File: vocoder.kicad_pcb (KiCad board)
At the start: 4 copper layers, 65.4 x 35.6 mm, 66 parts, among them J1 AudioJack4, J2 Conn_01x02_Socket, J3 Conn_01x02_Pin, J4 USB_C_Receptacle_USB2.0_16P, Q1 Q_NPN_BCE, Q2 Q_NPN_BCE, Q3 AO3401A, Q4 Q_NPN_BCE, SW1 SW_SPDT, SW2 SW_Push, SW3 SW_Push, U2 MAX98357A, U3 BQ24074RGT, U4 TPS63031DSK, U5 ADAU1761, U7 ESP32-S3-WROOM-1

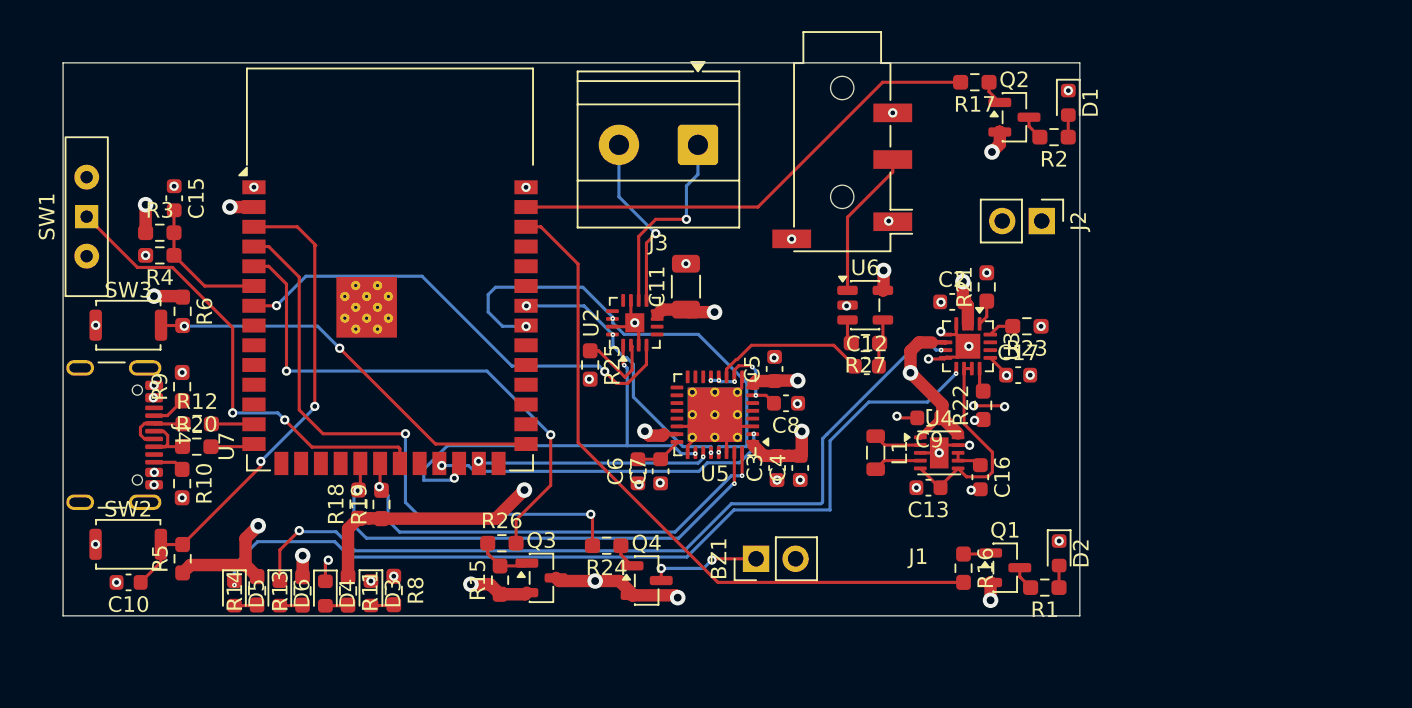
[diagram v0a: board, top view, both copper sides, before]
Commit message: semi working before removing battery and adding necessary changes
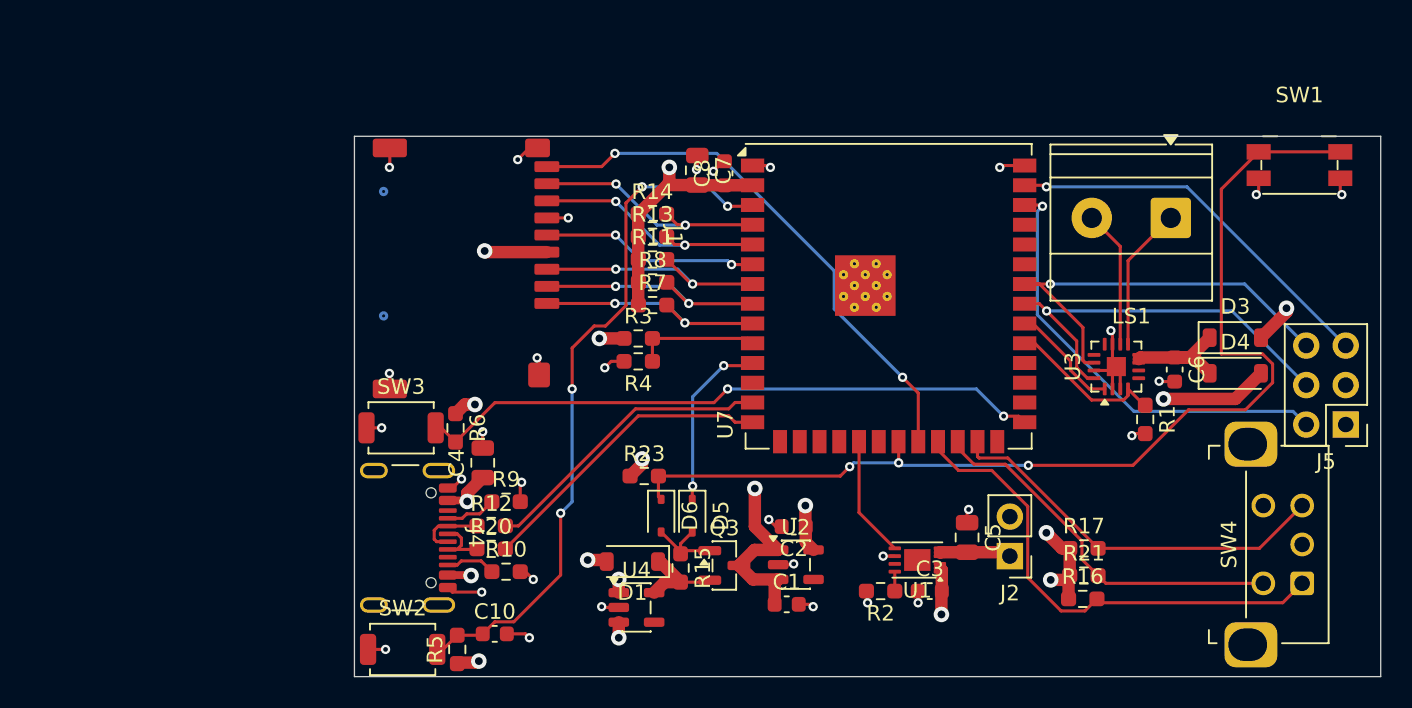
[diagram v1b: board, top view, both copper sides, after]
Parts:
- removed BZ1: Buzzer, Connector_PinHeader_2.54mm:PinHeader_1x02_P2.54mm_Vertical
- removed C11: 220u, Capacitor_SMD:C_1206_3216Metric
- removed C12: 2.2u, Capacitor_SMD:C_0603_1608Metric
- removed C13, C17, C9: 10u, Capacitor_SMD:C_0603_1608Metric
- removed C15: 100n, Capacitor_SMD:C_0603_1608Metric
- removed C16: 0.1u, Capacitor_SMD:C_0603_1608Metric
- removed D2: LED RED, LED_SMD:LED_0603_1608Metric
- removed J3: Conn_01x02_Pin, TerminalBlock_Phoenix:TerminalBlock_Phoenix_MKDS-1,5-2-5.08_1x02_P5.08mm_Horizontal
- removed L1: 1.5uH, Inductor_SMD:L_0805_2012Metric
- removed Q1, Q2, Q4: Q_NPN_BCE, Package_TO_SOT_SMD:SOT-23
- removed R18, R19: 10k, Resistor_SMD:R_0603_1608Metric_Pad0.98x0.95mm_HandSolder
- removed R22, R24: 1k, Resistor_SMD:R_0603_1608Metric_Pad0.98x0.95mm_HandSolder
- removed R25: 100k, Resistor_SMD:R_0603_1608Metric_Pad0.98x0.95mm_HandSolder
- removed R26: 100, Resistor_SMD:R_0603_1608Metric_Pad0.98x0.95mm_HandSolder
- removed R27: 51, Resistor_SMD:R_0603_1608Metric_Pad0.98x0.95mm_HandSolder
- removed U5: ADAU1761, Package_CSP:LFCSP-32-1EP_5x5mm_P0.5mm_EP3.5x3.5mm_ThermalVias
- removed U6: ~, custom_footprints:TLV9041
- added C1: 1u, Capacitor_SMD:C_0603_1608Metric, F.Cu at (169.6, 101.6)
- added J5: Conn_02x03_Top_Bottom, Connector_PinHeader_2.54mm:PinHeader_2x03_P2.54mm_Vertical, F.Cu at (205.5, 90.0)
- added LS1: Speaker, TerminalBlock_Phoenix:TerminalBlock_Phoenix_MKDS-1,5-2-5.08_1x02_P5.08mm_Horizontal, F.Cu at (194.2, 76.8)
- added R7: 10k, Resistor_SMD:R_0603_1608Metric_Pad0.98x0.95mm_HandSolder, F.Cu at (160.9, 82.4)
- added SW4: RotaryEncoder_Switch, Rotary_Encoder:RotaryEncoder_Bourns_Horizontal_PEC12R-2x17F-Sxxxx, F.Cu at (202.7, 100.2)
- added U1: MCP73831-2-MC, Package_DFN_QFN:DFN-8-1EP_3x2mm_P0.5mm_EP1.7x1.4mm, F.Cu at (177.9, 98.8)
- C2, C8: value 10u -> 1u
- C3, C6: value 100n -> 1u
- C4, C7: footprint Capacitor_SMD:C_0603_1608Metric -> Capacitor_SMD:C_0805_2012Metric
- C5: value 100n -> 10u; footprint Capacitor_SMD:C_0603_1608Metric -> Capacitor_SMD:C_0805_2012Metric
- D1: value LED RED -> SS34; footprint LED_SMD:LED_0603_1608Metric -> Diode_SMD:D_SOD-123
- D3: value LED BLUE -> SS34; footprint LED_SMD:LED_0603_1608Metric -> Diode_SMD:D_SOD-123
- D4: value LED GREEN -> SS34; footprint LED_SMD:LED_0603_1608Metric -> Diode_SMD:D_SOD-123
- D5: value LED RED -> 1N4148; footprint LED_SMD:LED_0603_1608Metric -> Diode_SMD:D_SOD-323
- D6: value LED GREEN -> 1N4148; footprint LED_SMD:LED_0603_1608Metric -> Diode_SMD:D_SOD-323
- J1: value AudioJack4 -> Micro_SD_Card_Det1; footprint Connector_Audio:Jack_3.5mm_PJ320D_Horizontal -> MyAntenna_manufacturer:Untitled
- R1, R11, R13, R14, R16, R17, R23, R8: value 1k -> 10k
- R2: value 1k -> 2.2k
- R3, R4: value 100k -> 470k
- SW1: value SW_SPDT -> SW_Push; footprint Button_Switch_THT:SW_Slide-03_Wuerth-WS-SLTV_10x2.5x6.4_P2.54mm -> Button_Switch_SMD:Panasonic_EVQPUJ_EVQPUA
- SW2, SW3: footprint Button_Switch_SMD:SW_Push_SPST_NO_Alps_SKRK -> Button_Switch_SMD:SW_SPST_TS-1088-xR020
- U2: value MAX98357A -> AP2112K-3.3; footprint Package_DFN_QFN:TQFN-16-1EP_3x3mm_P0.5mm_EP1.23x1.23mm -> Package_TO_SOT_SMD:SOT-23-5
- U3: value BQ24074RGT -> MAX98357A; footprint Package_DFN_QFN:VQFN-16-1EP_3x3mm_P0.5mm_EP1.6x1.6mm -> Package_DFN_QFN:TQFN-16-1EP_3x3mm_P0.5mm_EP1.23x1.23mm
- U4: value TPS63031DSK -> MAX40200AUK; footprint Package_SON:WSON-10-1EP_2.5x2.5mm_P0.5mm_EP1.2x2mm -> Package_TO_SOT_SMD:SOT-23-5
- U7: footprint RF_Module:ESP32-S3-WROOM-1 -> RF_Module:ESP32-S3-WROOM-1U
- moved SW1 78.1 mm to (202.5, 73.3), turned to 0 degrees
- moved D4 60.2 mm to (198.4, 86.7), turned to 0 degrees
- moved D3 58.0 mm to (198.4, 84.5), turned to 0 degrees
- moved D1 40.7 mm to (159.6, 98.8), turned to 180 degrees
- moved C6 35.1 mm to (194.5, 86.5), turned to -90 degrees
- moved R14 35.1 mm to (160.9, 76.5), turned to 0 degrees
- moved U7 32.1 mm to (176.1, 81.8)
- moved R13 32.0 mm to (160.9, 78.0), turned to 0 degrees
- moved R4 31.5 mm to (160.0, 86.0)
- moved R3 31.5 mm to (160.0, 84.5)
- moved R2 31.3 mm to (175.6, 100.8)
- moved R17 30.8 mm to (188.7, 98.0), turned to 0 degrees
- moved D5 29.9 mm to (163.5, 95.9)
- moved R11 28.9 mm to (160.9, 79.4), turned to 0 degrees
- moved R23 26.4 mm to (160.4, 93.3), turned to 0 degrees
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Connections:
- C2 pad 1: GND -> 3V3
- C2 pad 2: BATT+ -> GND
- C3 pad 2: 3V3 -> USB_5V
- C4 pad 1: GND -> USB_5V
- C4 pad 2: 3V3 -> GND
- C5 pad 1: 3V3 -> GND
- C5 pad 2: GND -> BATT+
- C6 pad 1: GND -> Net-(D3-K)
- C6 pad 2: Net-(U5-DVDDOUT) -> GND
- C7 pad 2: Net-(U5-DVDDOUT) -> 3V3
- C8 pad 1: GND -> 3V3
- C8 pad 2: CM -> GND
- D1 pad 1: GND -> Net-(D1-K)
- D1 pad 2: Net-(D1-A) -> USB_5V
- D3 pad 1: GND -> Net-(D3-K)
- D3 pad 2: Net-(D3-A) -> USB_5V
- D4 pad 1: GND -> Net-(D3-K)
- D4 pad 2: Net-(D4-A) -> AMP_POWER
- D5 pad 1: Net-(D5-K) -> POWER_SWITCH
- D6 pad 1: Net-(D6-K) -> BUTTON_READ
- D6 pad 2: Net-(D6-A) -> Net-(D5-A)
- Q3 pad 1: Net-(Q3-G) -> Net-(D5-A)
- Q3 pad 2: 3V3 -> Net-(D1-K)
- Q3 pad 3: 3V3_PRE -> AMP_POWER
- R1 pad 1: Net-(D2-A) -> AMP_SWITCH
- R1 pad 2: Net-(Q1-E) -> GND
- R11 pad 2: Net-(D4-A) -> CMD
- R13 pad 1: Net-(D6-A) -> 3V3
- R13 pad 2: 3V3_PRE -> D0
- R14 pad 1: Net-(D5-A) -> 3V3
- R14 pad 2: 3V3_PRE -> D1
- R15 pad 1: 3V3_PRE -> Net-(D5-A)
- R15 pad 2: Net-(Q3-G) -> Net-(D1-K)
- R16 pad 1: Net-(Q1-B) -> 3V3
- R16 pad 2: LED_RIGHT -> ENC_LEFT
- R17 pad 1: Net-(Q2-B) -> 3V3
- R17 pad 2: LED_LEFT -> ENC_RIGHT
- R2 pad 1: Net-(D1-A) -> Net-(U1-PROG)
- R2 pad 2: Net-(Q2-E) -> GND
- R21 pad 1: Net-(U3-TS) -> 3V3
- R21 pad 2: GND -> ENC_PUSH
- R23 pad 1: GND -> 3V3
- R23 pad 2: Net-(U3-ISET) -> BUTTON_READ
- R5 pad 1: 3V3_PRE -> 3V3
- R6 pad 1: 3V3_PRE -> 3V3
- R8 pad 1: USB_5V -> 3V3
- R8 pad 2: Net-(D3-A) -> D3
- SW1 pad 1: SWITCH_INPUT -> BUTTON_READ
- SW1 pad 2: 3V3_PRE -> GND
- U2 pad 1: I2S_DATA_OUT -> AMP_POWER
- U2 pad 2: Net-(U2-GAIN_SLOT) -> GND
- U2 pad 3: GND -> AMP_POWER
- U2 pad 4: AMP_SWITCH -> unconnected-(U2-NC-Pad4)
- U2 pad 5: unconnected-(U2-NC-Pad5) -> 3V3
- U3 pad 1: Net-(U3-TS) -> I2S_DATA_OUT
- U3 pad 10: Net-(U4-EN) -> Net-(U3-OUTN)
- U3 pad 11: Net-(U4-EN) -> GND
- U3 pad 12: Net-(U3-ILIM) -> unconnected-(U3-NC-Pad12)
- U3 pad 13: USB_5V -> unconnected-(U3-NC-Pad13)
- U3 pad 14: unconnected-(U3-TMR-Pad14) -> I2S_LRCLK
- U3 pad 15: unconnected-(U3-ITERM-Pad15) -> GND
- U3 pad 16: Net-(U3-ISET) -> I2S_BCLK
- U3 pad 2: BATT+ -> GND
- U3 pad 3: BATT+ -> GND
- U3 pad 4: GND -> AMP_SWITCH
- U3 pad 5: GND -> unconnected-(U3-NC-Pad5)
- U3 pad 6: 3V3_PRE -> unconnected-(U3-NC-Pad6)
- U3 pad 7: Net-(D6-K) -> Net-(D3-K)
- U3 pad 8: GND -> Net-(D3-K)
- U3 pad 9: Net-(D5-K) -> Net-(U3-OUTP)
- U4 pad 1: 3V3_PRE -> BATT+
- U4 pad 2: Net-(U4-L2) -> GND
- U4 pad 3: GND -> BATT+
- U4 pad 4: Net-(U4-L1) -> unconnected-(U4-NC-Pad4)
- U4 pad 5: Net-(U4-EN) -> Net-(D1-K)
- U7 pad 10: unconnected-(U7-IO17-Pad10) -> BATT_READ
- U7 pad 11: unconnected-(U7-IO18-Pad11) -> POWER_SWITCH
- U7 pad 19: SDA -> CHARGE_STATUS
- U7 pad 2: 3V3_PRE -> 3V3
- U7 pad 20: SCL -> unconnected-(U7-IO12-Pad20)
- U7 pad 21: SWITCH_INPUT -> BUTTON_READ
- U7 pad 22: unconnected-(U7-IO14-Pad22) -> DET
- U7 pad 23: I2S_MCLK -> ENC_LEFT
- U7 pad 24: I2S_DATA_OUT -> ENC_PUSH
- U7 pad 25: I2S_DATA_IN -> ENC_RIGHT
- U7 pad 31: unconnected-(U7-IO38-Pad31) -> AMP_SWITCH
- U7 pad 32: unconnected-(U7-IO39-Pad32) -> I2S_DATA_OUT
- U7 pad 33: I2S_LRCLK -> I2S_BCLK
- U7 pad 34: I2S_BCLK -> I2S_LRCLK
- U7 pad 38: LED_RIGHT -> I2S_MCLK
- U7 pad 39: LED_LEFT -> I2S_DATA_IN
- U7 pad 4: BUZZER -> D1
- U7 pad 5: 3V3_SWITCH -> D0
- U7 pad 6: BATT_READ -> CLK
- U7 pad 7: AMP_SWITCH -> CMD
- U7 pad 8: unconnected-(U7-IO15-Pad8) -> D3
- U7 pad 9: unconnected-(U7-IO16-Pad9) -> D2
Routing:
- net 3V3_PRE: track 145.5 -> 0.00 mm, vias 6 -> 0
- net BUTTON_READ: track 0.00 -> 69.1 mm, vias 0 -> 3
- net Net-(D5-K): track 56.8 -> 0.00 mm, vias 2 -> 0
- net Net-(D6-K): track 53.8 -> 0.00 mm, vias 2 -> 0
- net AMP_POWER: track 0.00 -> 47.7 mm, vias 0 -> 2
- net LED_RIGHT: track 44.3 -> 0.00 mm
- net BUZZER: track 38.5 -> 0.00 mm, vias 2 -> 0
- net DET: track 0.00 -> 35.2 mm, vias 0 -> 2
- net 3V3_SWITCH: track 34.7 -> 0.00 mm, vias 2 -> 0
- net SDA: track 32.4 -> 0.00 mm, vias 2 -> 0
- net ENC_LEFT: track 0.00 -> 31.9 mm
- net LED_LEFT: track 31.3 -> 0.00 mm
- net SCL: track 30.5 -> 0.00 mm, vias 2 -> 0
- net SWITCH_INPUT: track 30.5 -> 0.00 mm, vias 2 -> 0
- net ENC_RIGHT: track 0.00 -> 25.4 mm
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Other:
- board size 65.4 x 35.6 mm -> 66 x 34.8 mm
